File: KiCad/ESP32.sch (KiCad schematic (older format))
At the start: 1 part, among them U1 ESP32-DevKitC

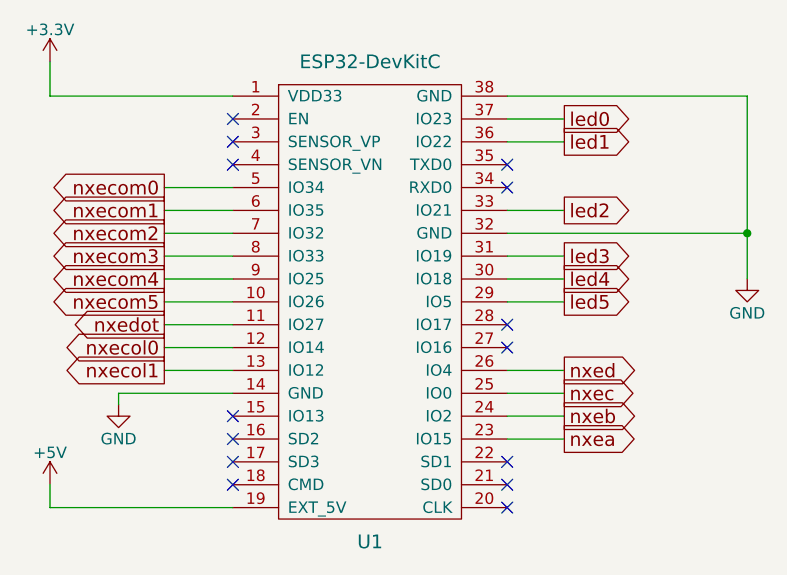
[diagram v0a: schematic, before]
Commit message: finish route
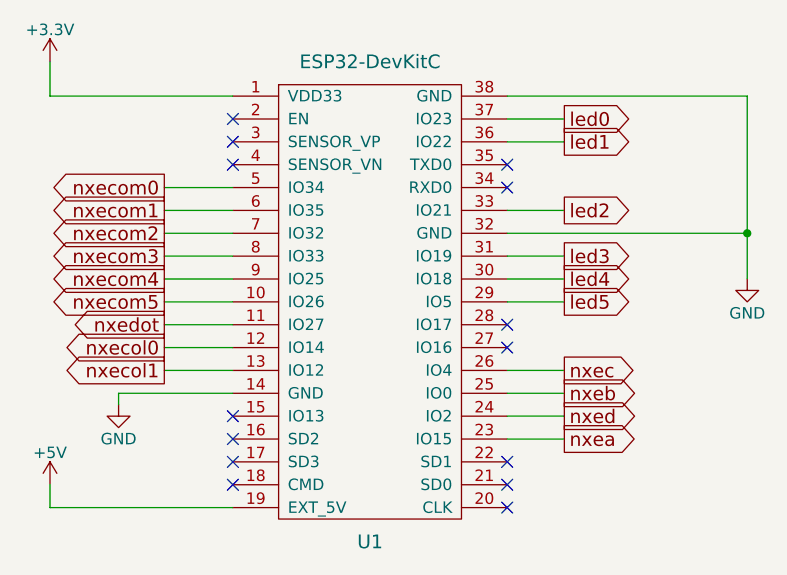
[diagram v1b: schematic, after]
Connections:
- net nxeb: now also U1.25 (IO0); no longer U1.24 (IO2)
- net nxec: now also U1.26 (IO4); no longer U1.25 (IO0)
- net nxed: now also U1.24 (IO2); no longer U1.26 (IO4)
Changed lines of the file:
@@
 Text GLabel 4000 3200 2    60   Output ~ 0
 nxea
+Text GLabel 4000 3000 2    60   Output ~ 0
+nxeb
+Text GLabel 4000 2900 2    60   Output ~ 0
+nxec
 Text GLabel 4000 3100 2    60   Output ~ 0
-nxeb
-Text GLabel 4000 3000 2    60   Output ~ 0
-nxec
-Text GLabel 4000 2900 2    60   Output ~ 0
 nxed
 Wire Wire Line
